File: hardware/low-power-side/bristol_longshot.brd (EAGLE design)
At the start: 36 x 44 mm, 68 parts, among them U1 SAM_D20E, U10 ADP1607ACPZN-R7, U11 TPS73118DBVT, U2 SI4060, U3 SE880, U4 SST25WF040BT-40I/NP, U5 TG-5006CJ, U6 TG-5006CJ, U7 TPS3123, U8 SN74LVC1G32DCKR, U9 MS5607-02BA03, Y1 ABS05

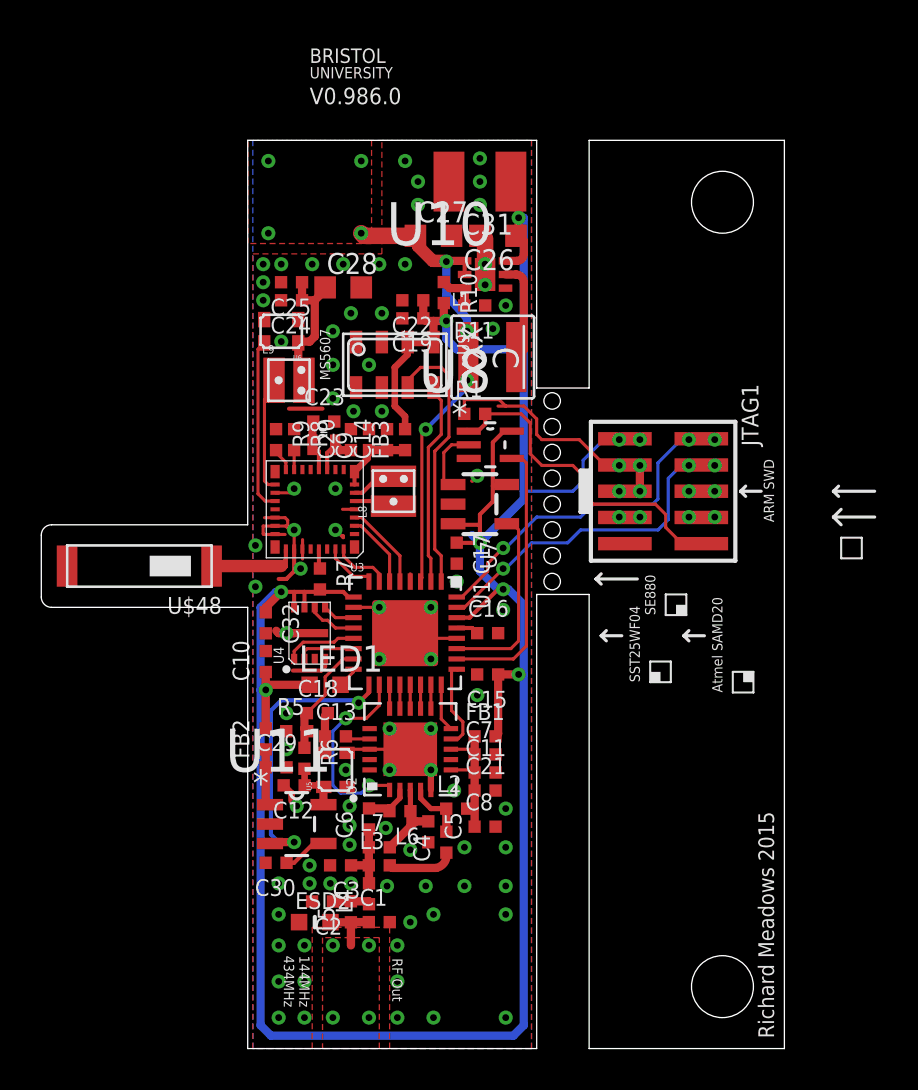
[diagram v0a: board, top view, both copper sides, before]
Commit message: [low-power-side] More work on board, vaguely complete. Added parts list
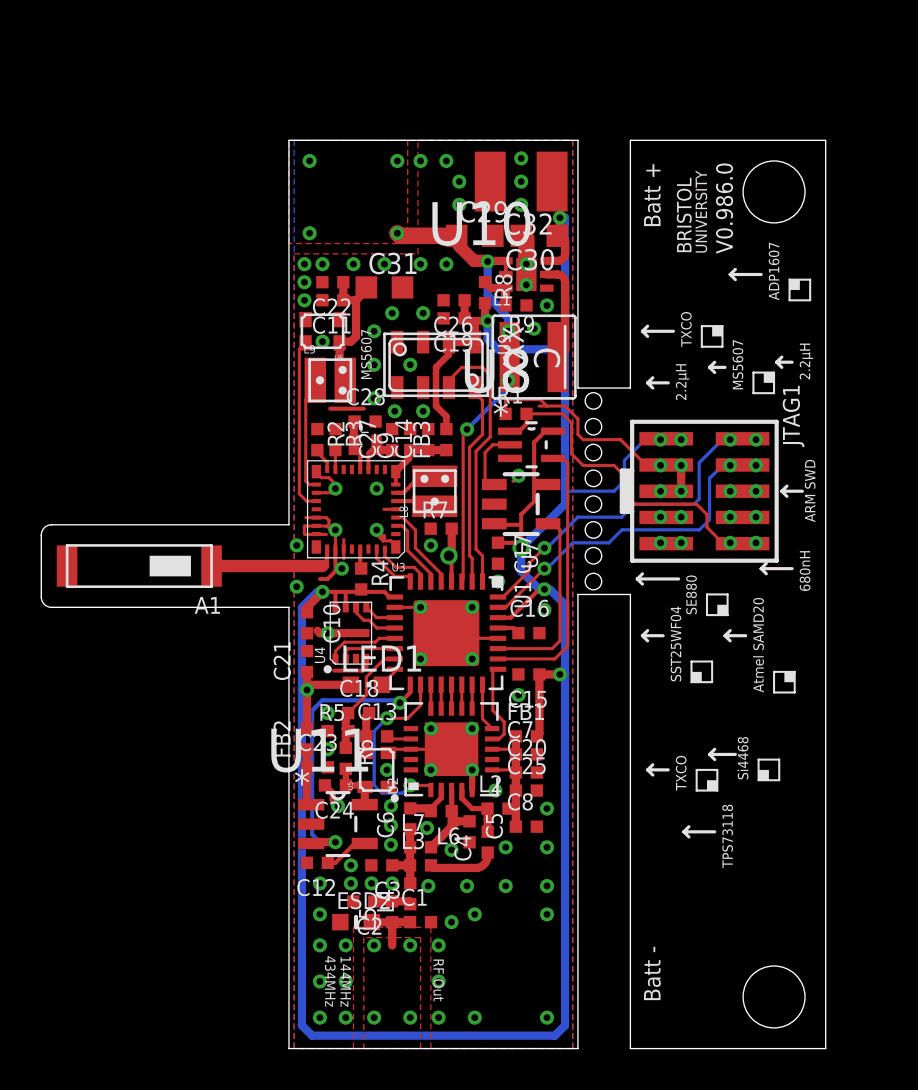
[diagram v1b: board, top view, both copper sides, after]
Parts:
- removed R10: 100kΩ, microbuilder_v3:_0402
- removed R11: 240kΩ, microbuilder_v3:_0402
- added R2, R3, R4: 10kΩ, microbuilder_v3:_0402
- C1, C13, C14, C15, C16, C17, C18, C19, C2, C3, C4, C5, C6, C7, C8, C9: device microbuilder_v3:_0402 -> microbuilder_v3:_0402@2
- C10: value 100nF -> 100pF; device microbuilder_v3:_0402 -> microbuilder_v3:_0402@2
- C11: value 100nF -> 1nF; device microbuilder_v3:_0402 -> microbuilder_v3:_0402@2
- C12: value 1µF -> 10nF; device microbuilder_v3:_0402 -> microbuilder_v3:_0402@2
- C20: value 18pF -> 100nF; device microbuilder_v3:_0402 -> microbuilder_v3:_0402@2
- C21: value 2.2µF -> 100nF; device microbuilder_v3:_0402 -> microbuilder_v3:_0402@2
- C22: value 4.7µF -> 100nF; device microbuilder_v3:_0402 -> microbuilder_v3:_0402@2
- C23: value 18pF -> 1µF; device microbuilder_v3:_0402 -> microbuilder_v3:_0402@2
- C24: value 1nF -> 1µF; device microbuilder_v3:_0402 -> microbuilder_v3:_0402@2
- C25: value 100nF -> 2.2µF; device microbuilder_v3:_0402 -> microbuilder_v3:_0402@2
- C26: value 10µF -> 4.7µF; device resistor:C0603K -> microbuilder_v3:_0402@2
- C27, C28: value 10µF -> 18pF; device resistor:C0603K -> microbuilder_v3:_0402@2
- C29: value 1µF -> 10µF; device microbuilder_v3:_0402 -> resistor:C0603K
- C30: value 10nF -> 10µF; device microbuilder_v3:_0402 -> resistor:C0603K
- C31: value 100µF -> 10µF; device resistor:C1210K -> resistor:C0603K
- C32: value 100pF -> 100µF; device microbuilder_v3:_0402 -> resistor:C1210K
- R7, R9: value 10kΩ -> 100kΩ
- R8: value 10kΩ -> 43kΩ
- moved C30 32.9 mm to (24.1, 39.4)
- moved C29 27.5 mm to (21.0, 39.4)
- moved C25 27.1 mm to (23.5, 12.5), turned to 0 degrees
- moved C32 24.7 mm to (23.2, 42.0), turned to 180 degrees
- moved C11 24.0 mm to (14.1, 36.2), turned to 180 degrees
- moved C24 23.6 mm to (14.2, 12.8)
- moved C20 18.2 mm to (23.5, 13.4), turned to 0 degrees
- moved C23 16.8 mm to (13.4, 13.6)
- moved R9 13.3 mm to (23.0, 36.0), turned to 180 degrees
- moved R8 11.7 mm to (21.5, 36.6)
- moved C21 10.7 mm to (12.9, 18.8), turned to 90 degrees
- moved C27 10.1 mm to (17.0, 29.5), turned to 90 degrees
- moved C31 6.90 mm to (16.6, 36.9), turned to 0 degrees
- moved C28 6.59 mm to (15.7, 30.4)
- moved R7 6.36 mm to (19.4, 25.2), turned to 0 degrees
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- renumbered U$48 to A1
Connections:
- removed net GPS!RESET: U1.4
- new net EXT_THERMISTOR_SENSE: R7.2, U1.4
- net 1.2V: now also C29.1; no longer C27.1
- net 1.8V: now also C21.1, C30.1, R4.2, R8.2; no longer C22.1, C31.1, R10.2, R7.2
- net FB: now also R8.1, R9.2; no longer R10.1, R11.2
- net GND: now also R2.1, R3.1, R7.1; no longer R11.1, R8.1
- net RADIO_VDD: now also C20.1, C25.1; no longer C11.1, C21.1
- net RTC_XI: now also C27.1; no longer C20.1
- net RTC_XO: now also C28.1; no longer C23.1
- net SE_GPIO0: now also R2.2; no longer R9.2
- net SE_GPIO1: now also R3.2; no longer R8.2
- net SE_MODE_PULL: now also R4.1; no longer R7.1
- net TCXO_REG_IN: now also C23.1; no longer C29.1
- net TCXO_REG_NR: now also C12.1; no longer C30.1
- net TCXO_VDD: now also C24.1; no longer C12.1
- net TCXO_VDD1: now also C11.1, C22.1, C31.1; no longer C24.1, C25.1, C28.1
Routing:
- net EXT_THERMISTOR_SENSE: track 0.00 -> 2.67 mm, vias 0 -> 1
- net GND: track 44.6 -> 47.2 mm, vias 88 -> 90
- net GPS_ANT: track 4.93 -> 6.93 mm
- net EXT!RESET: track 16.4 -> 17.3 mm, vias 0 -> 2
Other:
- board size 36 x 44 mm -> 38 x 44 mm
- board text added: "2.2µH"
- board text added: "680nH"
- board text added: "ADP1607"
- board text added: "Batt +"
- board text added: "Batt -"
- board text added: "Si4468"
- board text added: "TPS73118"
- board text added: "TXCO"
